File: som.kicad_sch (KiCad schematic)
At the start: 34 parts, among them M1 jetson-orin-nx/nano-module, U4 NTS0102GT

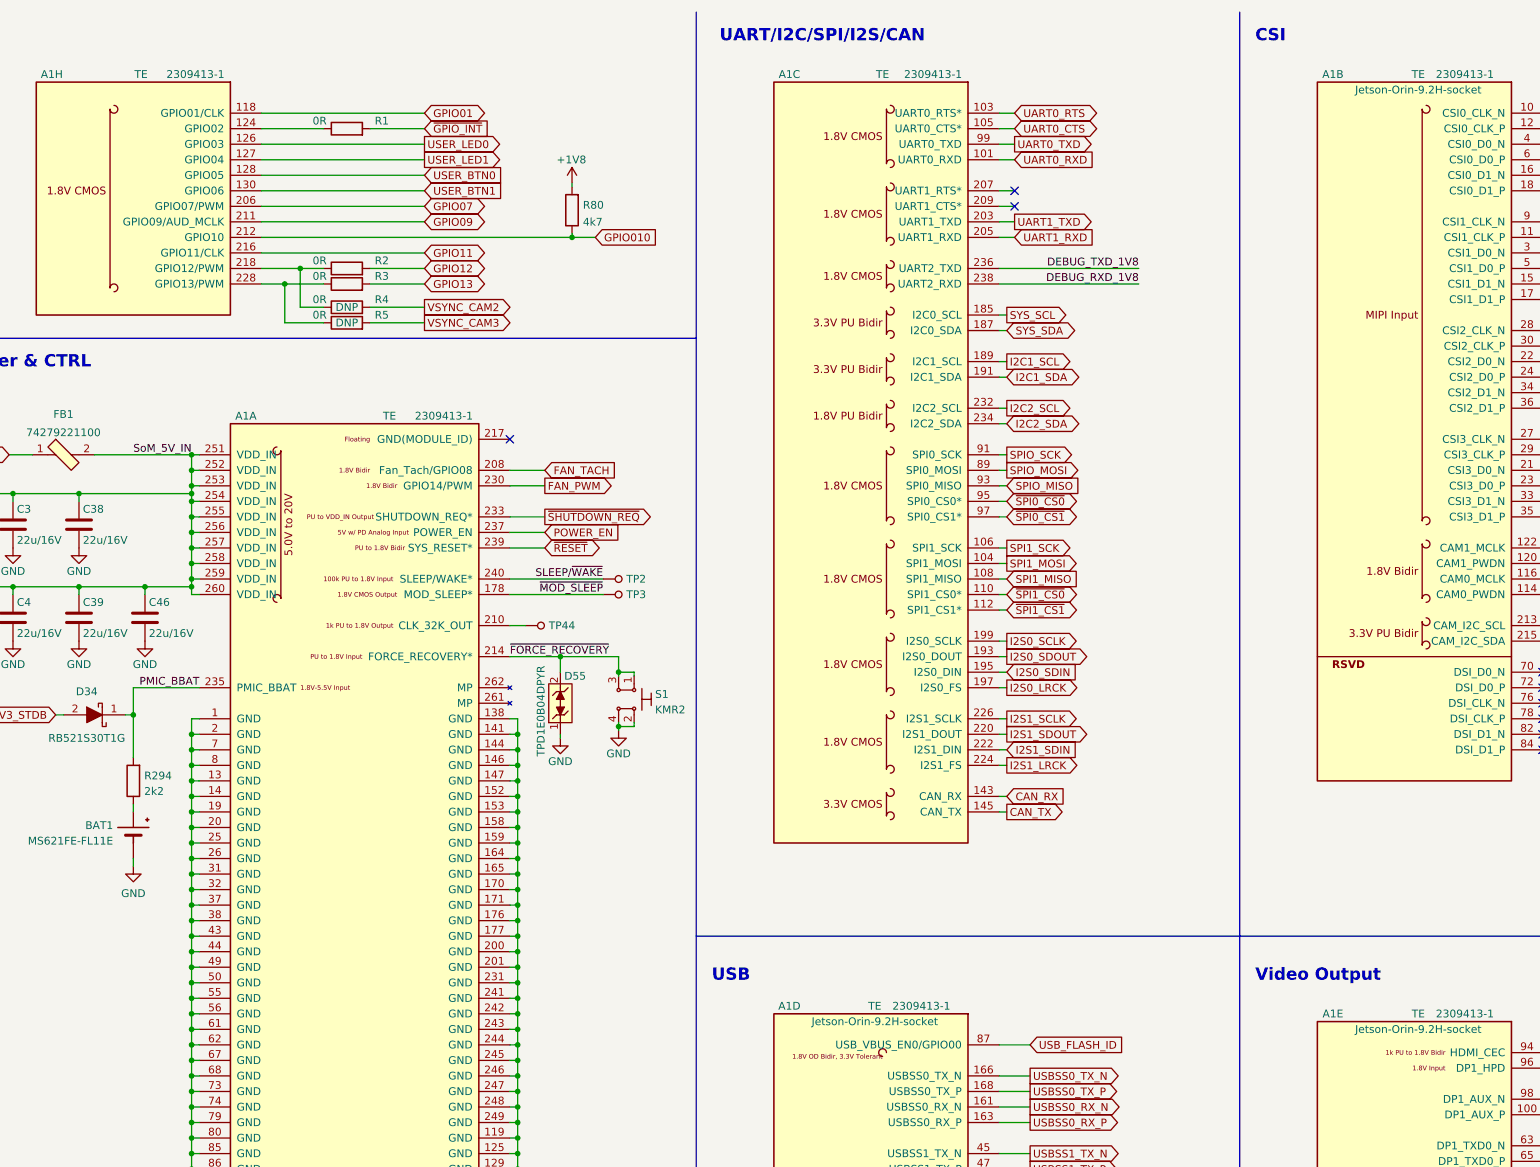
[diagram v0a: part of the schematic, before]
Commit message: Simplification continues
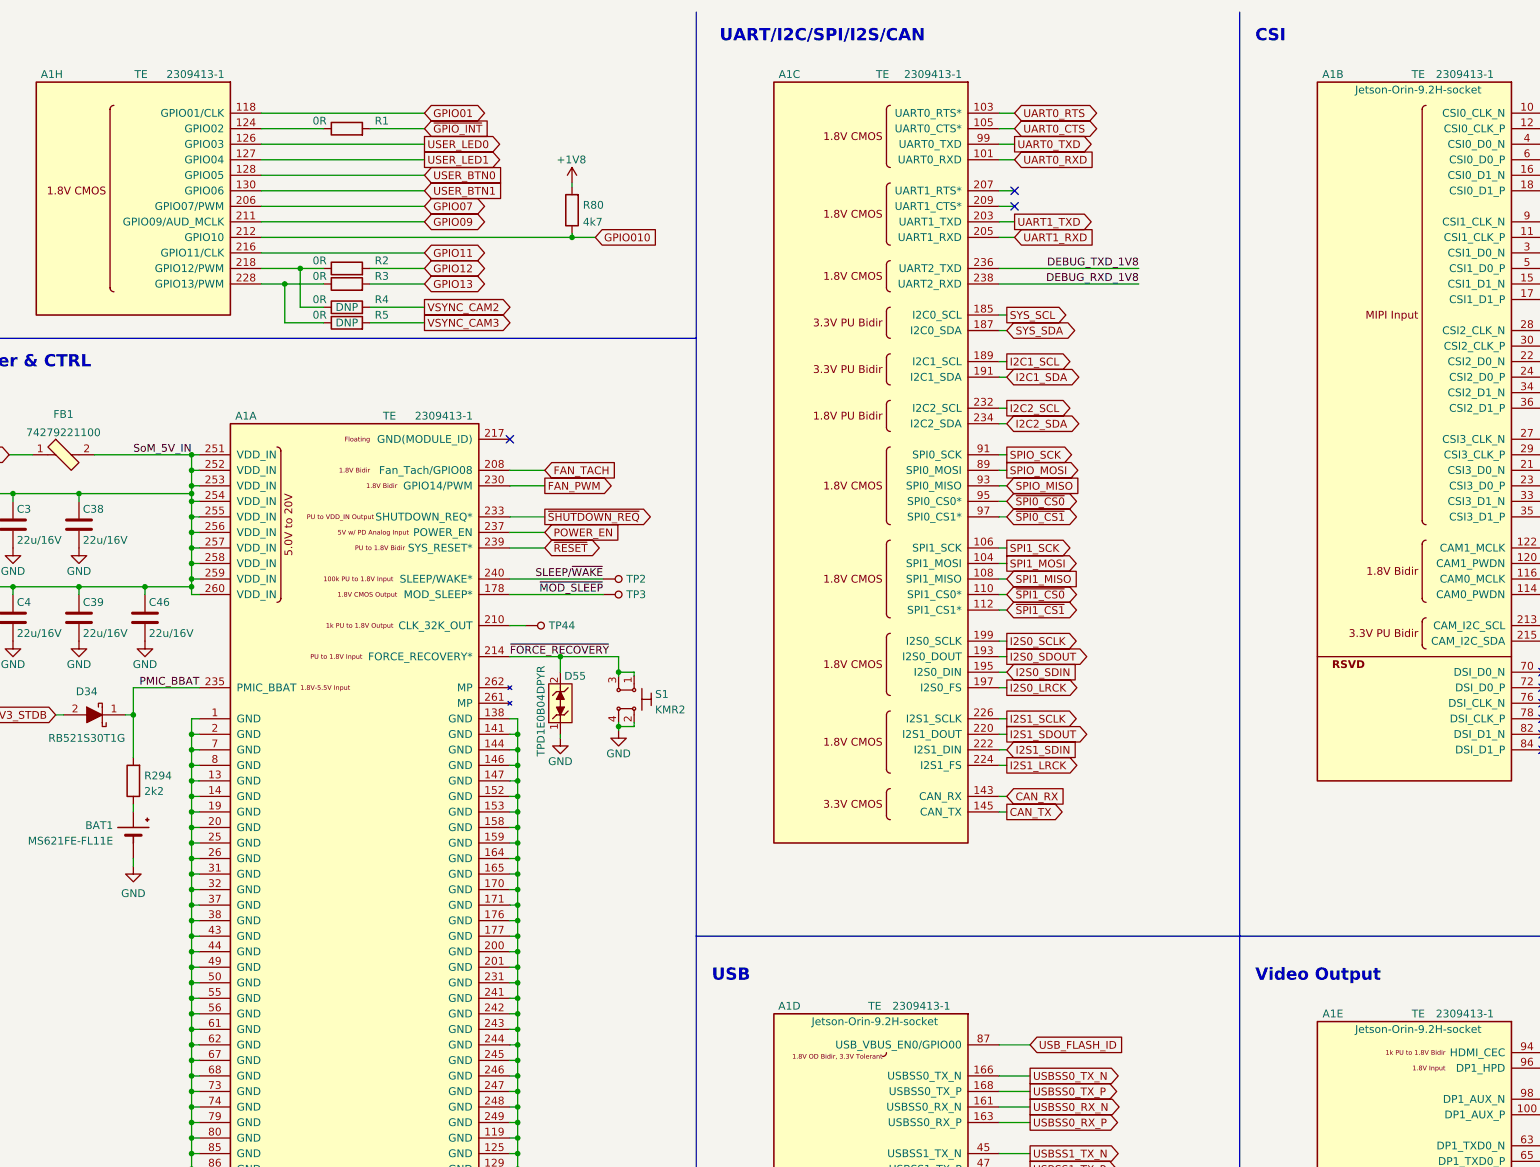
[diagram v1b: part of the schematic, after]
